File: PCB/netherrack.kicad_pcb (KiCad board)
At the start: 4 copper layers, 100 x 100 mm, 67 parts, among them J1 Conn_01x04, J11 USB_C_Receptacle_USB2.0, J12 USB3_A, J14 JST_SHBM04B-SRSS-TB, J2 Conn_02x07_Odd_Even, J22 690-019-298-412, J4 Bus_M.2_Socket_M, J6 THD-02-R, J7 Micro_SD_Card_Det, J9 THD-02-R, SW1 Right angle Tact button, U1 TPD4EUSB30, U12 RT9742SNGV, U18 RT9742GGJ5, U2 TPD4EUSB30, U3 MagJack-A70-112-331N126, U6 AP22653W6, U7 ASEK-32.768KHZ-L-R-T, U8 AP3441SHE-7B

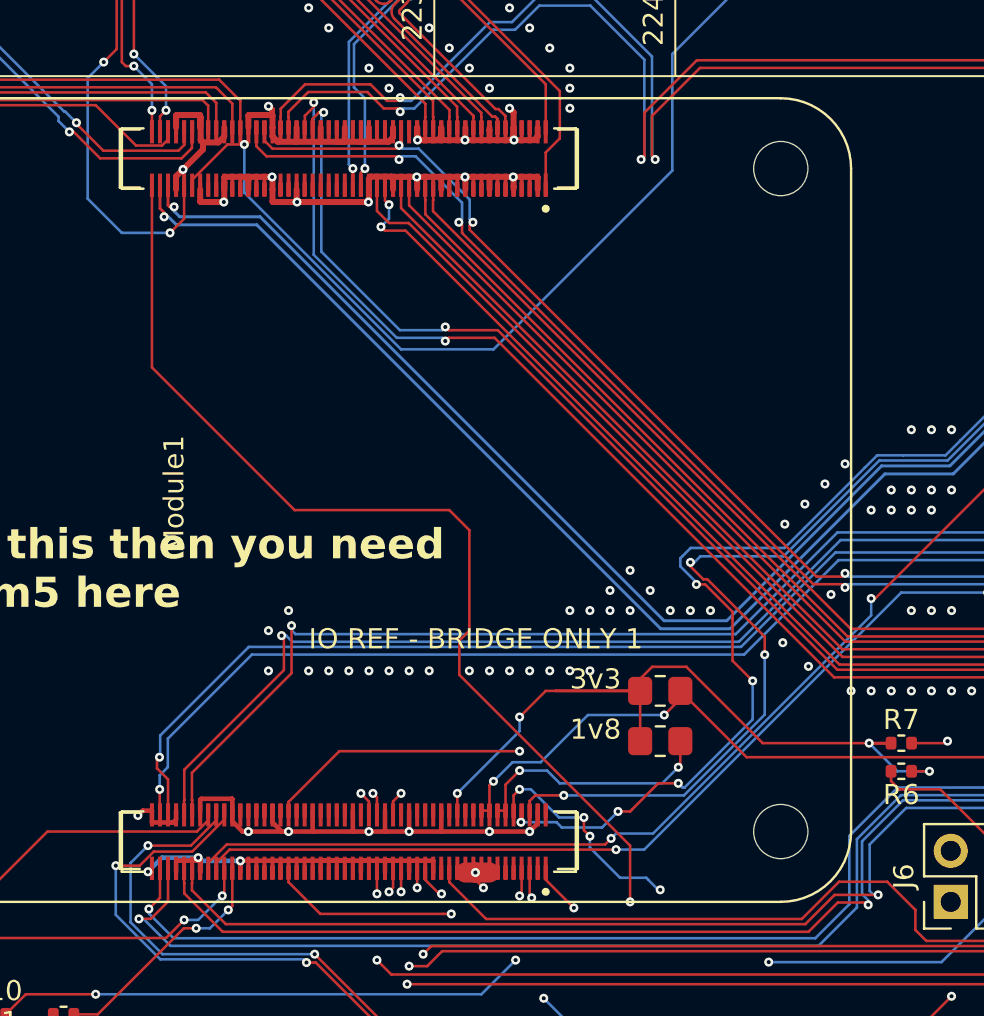
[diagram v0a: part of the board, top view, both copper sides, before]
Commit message: Update completed PCB
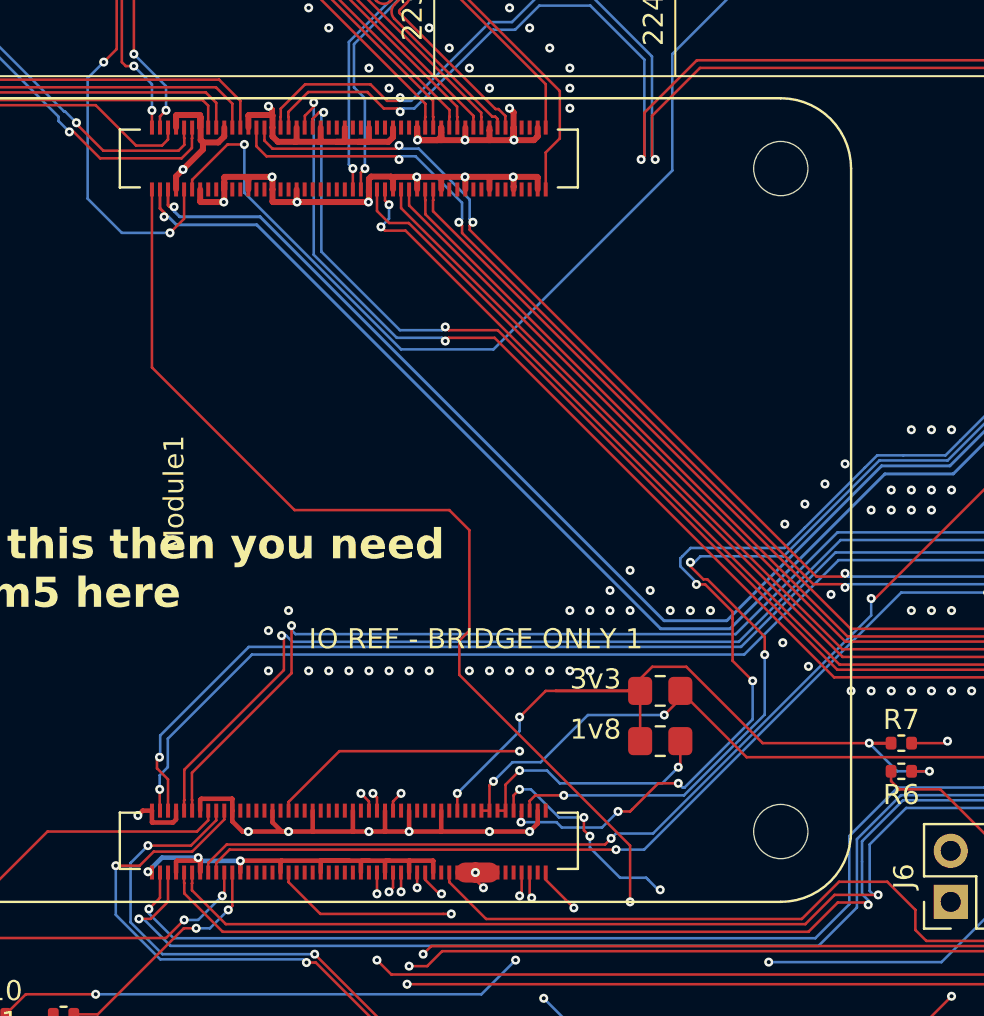
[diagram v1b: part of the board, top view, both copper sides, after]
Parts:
- removed REF** (x2): AMPHENOL_10164227-1001A1RLF, cm5conn:AMPHENOL_10164227-1001A1RLF

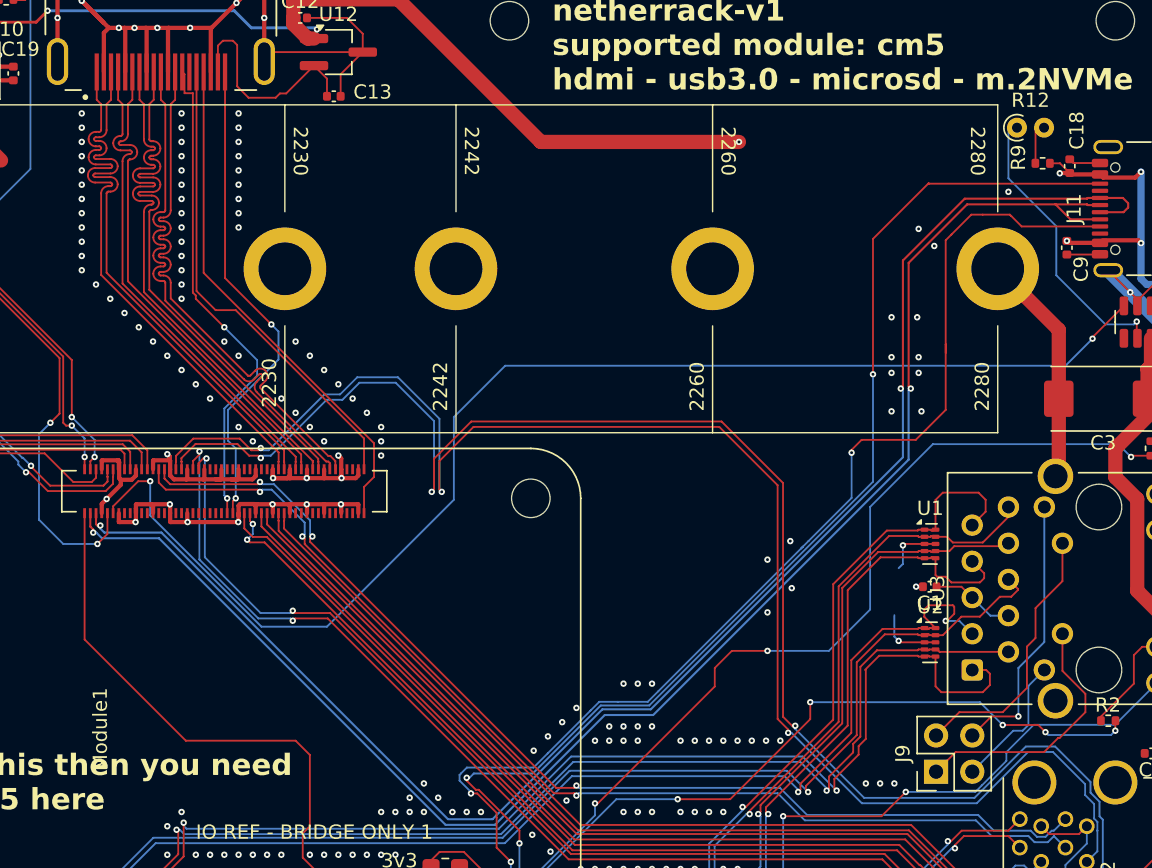
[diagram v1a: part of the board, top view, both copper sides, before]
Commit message: Submission commit
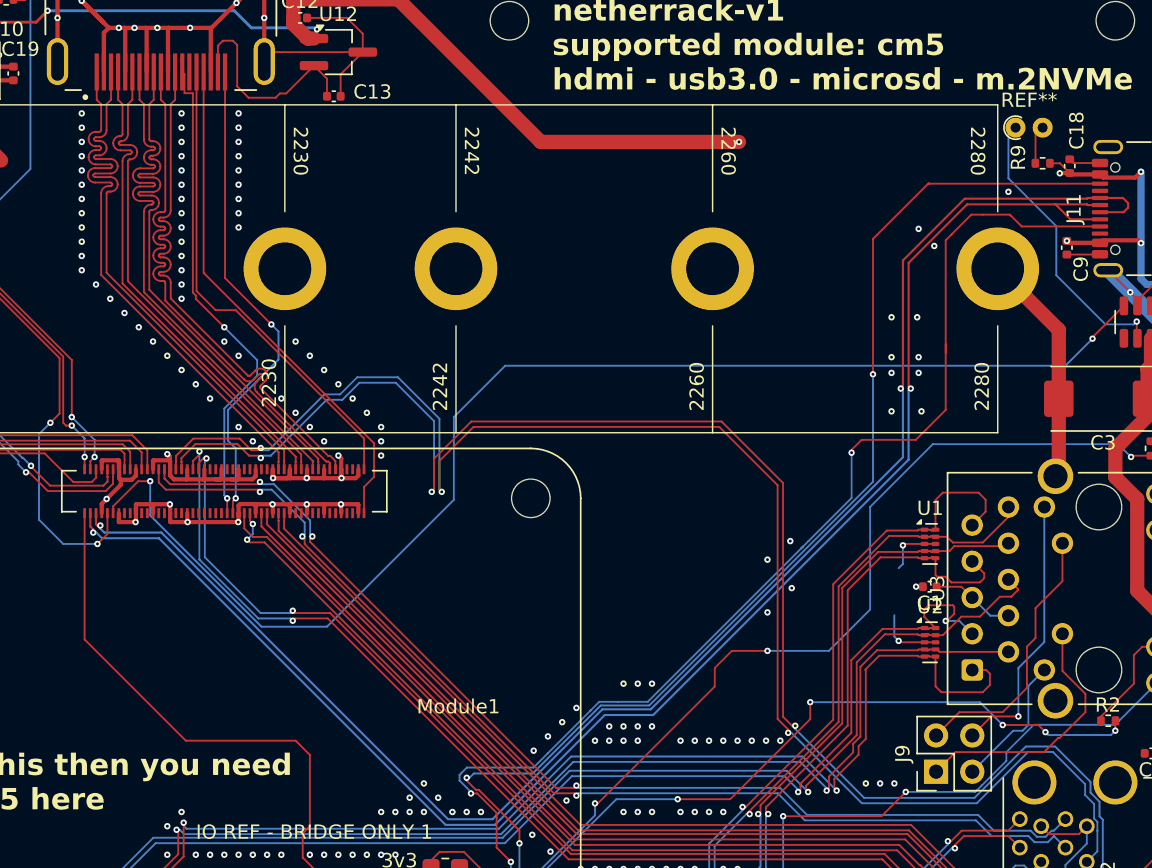
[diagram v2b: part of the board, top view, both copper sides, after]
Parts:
- removed R12: 15K 1%, Resistor_THT:R_Axial_DIN0204_L3.6mm_D1.6mm_P1.90mm_Vertical
- added REF**: R_Axial_DIN0204_L3.6mm_D1.6mm_P1.90mm_Vertical, Resistor_THT:R_Axial_DIN0204_L3.6mm_D1.6mm_P1.90mm_Vertical, F.Cu at (160.5, 60.0)
- D3: value LED Green -> LED
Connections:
- Module1 pad 1: (no net) -> GND
- Module1 pad 10: (no net) -> /GPIO (Ethernet, SD_CARD for CM5L)/TRD0_N
- Module1 pad 100: (no net) -> /GPIO (Ethernet, SD_CARD for CM5L)/CAM_GPIO1
- Module1 pad 101: (no net) -> /GPIO (Ethernet, SD_CARD for CM5L)/USBOTG
- Module1 pad 102: (no net) -> /Highspeed (USB, HDMI)/PCIE_nCLKREQ
- Module1 pad 103: (no net) -> /USB2_N
- Module1 pad 104: (no net) -> /Highspeed (USB, HDMI)/PCIE_nWAKE
- Module1 pad 105: (no net) -> /USB2_P
- Module1 pad 106: (no net) -> /Highspeed (USB, HDMI)/PCIE_PWR_EN
- Module1 pad 107: (no net) -> GND
- Module1 pad 108: (no net) -> GND
- Module1 pad 109: (no net) -> /Highspeed (USB, HDMI)/PCIE_nRST
- Module1 pad 11: (no net) -> /GPIO (Ethernet, SD_CARD for CM5L)/TRD2_P
- Module1 pad 110: (no net) -> /Highspeed (USB, HDMI)/PCIE_CLK_P
- Module1 pad 111: (no net) -> /Highspeed (USB, HDMI)/VBUS_EN
- Module1 pad 112: (no net) -> /Highspeed (USB, HDMI)/PCIE_CLK_N
- Module1 pad 113: (no net) -> GND
- Module1 pad 114: (no net) -> GND
- Module1 pad 115: (no net) -> /Highspeed (USB, HDMI)/DPHY0_D0_N
- Module1 pad 116: (no net) -> /Highspeed (USB, HDMI)/PCIE_RX_P
- Module1 pad 117: (no net) -> /Highspeed (USB, HDMI)/DPHY0_D0_P
- Module1 pad 118: (no net) -> /Highspeed (USB, HDMI)/PCIE_RX_N
- Module1 pad 119: (no net) -> GND
- Module1 pad 12: (no net) -> /GPIO (Ethernet, SD_CARD for CM5L)/TRD0_P
- Module1 pad 120: (no net) -> GND
- Module1 pad 121: (no net) -> /Highspeed (USB, HDMI)/DPHY0_D1_N
- Module1 pad 122: (no net) -> /Highspeed (USB, HDMI)/PCIE_TX_P
- Module1 pad 123: (no net) -> /Highspeed (USB, HDMI)/DPHY0_D1_P
- Module1 pad 124: (no net) -> /Highspeed (USB, HDMI)/PCIE_TX_N
- Module1 pad 125: (no net) -> GND
- Module1 pad 126: (no net) -> GND
- Module1 pad 127: (no net) -> /Highspeed (USB, HDMI)/DPHY0_C_N
- Module1 pad 128: (no net) -> /Highspeed (USB, HDMI)/USB3-0-RX_N
- Module1 pad 129: (no net) -> /Highspeed (USB, HDMI)/DPHY0_C_P
- Module1 pad 13: (no net) -> GND
- Module1 pad 130: (no net) -> /Highspeed (USB, HDMI)/USB3-0-RX_P
- Module1 pad 131: (no net) -> GND
- Module1 pad 132: (no net) -> GND
- Module1 pad 133: (no net) -> /Highspeed (USB, HDMI)/DPHY0_D2_N
- Module1 pad 134: (no net) -> /Highspeed (USB, HDMI)/USB3-0-D_P
- Module1 pad 135: (no net) -> /Highspeed (USB, HDMI)/DPHY0_D2_P
- Module1 pad 136: (no net) -> /Highspeed (USB, HDMI)/USB3-0-D_N
- Module1 pad 137: (no net) -> GND
- Module1 pad 138: (no net) -> GND
- Module1 pad 139: (no net) -> /Highspeed (USB, HDMI)/DPHY0_D3_N
- Module1 pad 14: (no net) -> GND
- Module1 pad 140: (no net) -> /Highspeed (USB, HDMI)/USB3-0-TX_N
- Module1 pad 141: (no net) -> /Highspeed (USB, HDMI)/DPHY0_D3_P
- Module1 pad 142: (no net) -> /Highspeed (USB, HDMI)/USB3-0-TX_P
- Module1 pad 143: (no net) -> /Highspeed (USB, HDMI)/HDMI1_HOTPLUG
- Module1 pad 144: (no net) -> GND
- Module1 pad 145: (no net) -> /Highspeed (USB, HDMI)/HDMI1_SDA
- Module1 pad 146: (no net) -> /Highspeed (USB, HDMI)/HDMI1_D2_P
- Module1 pad 147: (no net) -> /Highspeed (USB, HDMI)/HDMI1_SCL
- Module1 pad 148: (no net) -> /Highspeed (USB, HDMI)/HDMI1_D2_N
- Module1 pad 149: (no net) -> /Highspeed (USB, HDMI)/HDMI1_CEC
- Module1 pad 15: (no net) -> /GPIO (Ethernet, SD_CARD for CM5L)/ETH_LEDY
- Module1 pad 150: (no net) -> GND
- Module1 pad 151: (no net) -> /Highspeed (USB, HDMI)/HDMI0_CEC
- Module1 pad 152: (no net) -> /Highspeed (USB, HDMI)/HDMI1_D1_P
- Module1 pad 153: (no net) -> /Highspeed (USB, HDMI)/HDMI0_HOTPLUG
- Module1 pad 154: (no net) -> /Highspeed (USB, HDMI)/HDMI1_D1_N
- Module1 pad 155: (no net) -> GND
- Module1 pad 156: (no net) -> GND
- Module1 pad 157: (no net) -> /Highspeed (USB, HDMI)/USB3-1-RX_N
- Module1 pad 158: (no net) -> /Highspeed (USB, HDMI)/HDMI1_D0_P
- Module1 pad 159: (no net) -> /Highspeed (USB, HDMI)/USB3-1-RX_P
- Module1 pad 16: (no net) -> /GPIO (Ethernet, SD_CARD for CM5L)/TACHO
- Module1 pad 160: (no net) -> /Highspeed (USB, HDMI)/HDMI1_D0_N
- Module1 pad 161: (no net) -> GND
- Module1 pad 162: (no net) -> GND
- Module1 pad 163: (no net) -> /Highspeed (USB, HDMI)/USB3-1-D_P
- Module1 pad 164: (no net) -> /Highspeed (USB, HDMI)/HDMI1_CK_P
- Module1 pad 165: (no net) -> /Highspeed (USB, HDMI)/USB3-1-D_N
- Module1 pad 166: (no net) -> /Highspeed (USB, HDMI)/HDMI1_CK_N
- Module1 pad 167: (no net) -> GND
- Module1 pad 168: (no net) -> GND
- Module1 pad 169: (no net) -> /Highspeed (USB, HDMI)/USB3-1-TX_N
- Module1 pad 17: (no net) -> /GPIO (Ethernet, SD_CARD for CM5L)/ETH_LEDG
- Module1 pad 170: (no net) -> /Highspeed (USB, HDMI)/HDMI0_D2_P
- Module1 pad 171: (no net) -> /Highspeed (USB, HDMI)/USB3-1-TX_P
- Module1 pad 172: (no net) -> /Highspeed (USB, HDMI)/HDMI0_D2_N
- Module1 pad 173: (no net) -> GND
- Module1 pad 174: (no net) -> GND
- Module1 pad 175: (no net) -> /Highspeed (USB, HDMI)/DPHY1_D0_N
- Module1 pad 176: (no net) -> /Highspeed (USB, HDMI)/HDMI0_D1_P
- Module1 pad 177: (no net) -> /Highspeed (USB, HDMI)/DPHY1_D0_P
- Module1 pad 178: (no net) -> /Highspeed (USB, HDMI)/HDMI0_D1_N
- Module1 pad 179: (no net) -> GND
- Module1 pad 18: (no net) -> /GPIO (Ethernet, SD_CARD for CM5L)/SYNC_OUT
- Module1 pad 180: (no net) -> GND
- Module1 pad 181: (no net) -> /Highspeed (USB, HDMI)/DPHY1_D1_N
- Module1 pad 182: (no net) -> /Highspeed (USB, HDMI)/HDMI0_D0_P
- Module1 pad 183: (no net) -> /Highspeed (USB, HDMI)/DPHY1_D1_P
- Module1 pad 184: (no net) -> /Highspeed (USB, HDMI)/HDMI0_D0_N
- Module1 pad 185: (no net) -> GND
- Module1 pad 186: (no net) -> GND
- Module1 pad 187: (no net) -> /Highspeed (USB, HDMI)/DPHY1_C_N
- Module1 pad 188: (no net) -> /Highspeed (USB, HDMI)/HDMI0_CK_P
- Module1 pad 189: (no net) -> /Highspeed (USB, HDMI)/DPHY1_C_P
- Module1 pad 19: (no net) -> /GPIO (Ethernet, SD_CARD for CM5L)/PWM
- Module1 pad 190: (no net) -> /Highspeed (USB, HDMI)/HDMI0_CK_N
- Module1 pad 191: (no net) -> GND
- Module1 pad 192: (no net) -> GND
- Module1 pad 193: (no net) -> /Highspeed (USB, HDMI)/DPHY1_D2_N
- Module1 pad 194: (no net) -> /Highspeed (USB, HDMI)/DPHY1_D3_N
- Module1 pad 195: (no net) -> /Highspeed (USB, HDMI)/DPHY1_D2_P
- Module1 pad 196: (no net) -> /Highspeed (USB, HDMI)/DPHY1_D3_P
- Module1 pad 197: (no net) -> GND
- Module1 pad 198: (no net) -> GND
- Module1 pad 199: (no net) -> /Highspeed (USB, HDMI)/HDMI0_SDA
- Module1 pad 2: (no net) -> GND
- Module1 pad 20: (no net) -> /GPIO (Ethernet, SD_CARD for CM5L)/EEPROM_nWP
- Module1 pad 200: (no net) -> /Highspeed (USB, HDMI)/HDMI0_SCL
- Module1 pad 21: (no net) -> Net-(Module1A-LED_nACT)
- Module1 pad 22: (no net) -> GND
- Module1 pad 23: (no net) -> GND
- Module1 pad 24: (no net) -> /GPIO (Ethernet, SD_CARD for CM5L)/GPIO26
- Module1 pad 25: (no net) -> /GPIO (Ethernet, SD_CARD for CM5L)/GPIO21
- Module1 pad 26: (no net) -> /GPIO (Ethernet, SD_CARD for CM5L)/GPIO19
- Module1 pad 27: (no net) -> /GPIO (Ethernet, SD_CARD for CM5L)/GPIO20
- Module1 pad 28: (no net) -> /GPIO (Ethernet, SD_CARD for CM5L)/GPIO13
- Module1 pad 29: (no net) -> /GPIO (Ethernet, SD_CARD for CM5L)/GPIO16
- Module1 pad 3: (no net) -> /GPIO (Ethernet, SD_CARD for CM5L)/TRD3_P
- Module1 pad 30: (no net) -> /GPIO (Ethernet, SD_CARD for CM5L)/GPIO6
- Module1 pad 31: (no net) -> /GPIO (Ethernet, SD_CARD for CM5L)/GPIO12
- Module1 pad 32: (no net) -> GND
- Module1 pad 33: (no net) -> GND
- Module1 pad 34: (no net) -> /GPIO (Ethernet, SD_CARD for CM5L)/GPIO5
- Module1 pad 35: (no net) -> /GPIO (Ethernet, SD_CARD for CM5L)/ID_SC
- Module1 pad 36: (no net) -> /GPIO (Ethernet, SD_CARD for CM5L)/ID_SD
- Module1 pad 37: (no net) -> /GPIO (Ethernet, SD_CARD for CM5L)/GPIO7
- Module1 pad 38: (no net) -> /GPIO (Ethernet, SD_CARD for CM5L)/GPIO11
- Module1 pad 39: (no net) -> /GPIO (Ethernet, SD_CARD for CM5L)/GPIO8
- Module1 pad 4: (no net) -> /GPIO (Ethernet, SD_CARD for CM5L)/TRD1_P
- Module1 pad 40: (no net) -> /GPIO (Ethernet, SD_CARD for CM5L)/GPIO9
- Module1 pad 41: (no net) -> /GPIO (Ethernet, SD_CARD for CM5L)/GPIO25
- Module1 pad 42: (no net) -> GND
- Module1 pad 43: (no net) -> GND
- Module1 pad 44: (no net) -> /GPIO (Ethernet, SD_CARD for CM5L)/GPIO10
- Module1 pad 45: (no net) -> /GPIO (Ethernet, SD_CARD for CM5L)/GPIO24
- Module1 pad 46: (no net) -> /GPIO (Ethernet, SD_CARD for CM5L)/GPIO22
- Module1 pad 47: (no net) -> /GPIO (Ethernet, SD_CARD for CM5L)/GPIO23
- Module1 pad 48: (no net) -> /GPIO (Ethernet, SD_CARD for CM5L)/GPIO27
- Module1 pad 49: (no net) -> /GPIO (Ethernet, SD_CARD for CM5L)/GPIO18
- Module1 pad 5: (no net) -> /GPIO (Ethernet, SD_CARD for CM5L)/TRD3_N
- Module1 pad 50: (no net) -> /GPIO (Ethernet, SD_CARD for CM5L)/GPIO17
- Module1 pad 51: (no net) -> /GPIO (Ethernet, SD_CARD for CM5L)/GPIO15
- Module1 pad 52: (no net) -> GND
- Module1 pad 53: (no net) -> GND
- Module1 pad 54: (no net) -> /GPIO (Ethernet, SD_CARD for CM5L)/GPIO4
- Module1 pad 55: (no net) -> /GPIO (Ethernet, SD_CARD for CM5L)/GPIO14
- Module1 pad 56: (no net) -> /GPIO (Ethernet, SD_CARD for CM5L)/GPIO3
- Module1 pad 57: (no net) -> /GPIO (Ethernet, SD_CARD for CM5L)/SD_CLK
- Module1 pad 58: (no net) -> /GPIO (Ethernet, SD_CARD for CM5L)/GPIO2
- Module1 pad 59: (no net) -> GND
- Module1 pad 6: (no net) -> /GPIO (Ethernet, SD_CARD for CM5L)/TRD1_N
- Module1 pad 60: (no net) -> GND
- Module1 pad 61: (no net) -> /GPIO (Ethernet, SD_CARD for CM5L)/SD_DAT3
- Module1 pad 62: (no net) -> /GPIO (Ethernet, SD_CARD for CM5L)/SD_CMD
- Module1 pad 63: (no net) -> /GPIO (Ethernet, SD_CARD for CM5L)/SD_DAT0
- Module1 pad 64: (no net) -> unconnected-(Module1A-SD_DAT5-Pad64)
- Module1 pad 65: (no net) -> GND
- Module1 pad 66: (no net) -> GND
- Module1 pad 67: (no net) -> /GPIO (Ethernet, SD_CARD for CM5L)/SD_DAT1
- Module1 pad 68: (no net) -> unconnected-(Module1A-SD_DAT4-Pad68)
- Module1 pad 69: (no net) -> /GPIO (Ethernet, SD_CARD for CM5L)/SD_DAT2
- Module1 pad 7: (no net) -> GND
- Module1 pad 70: (no net) -> unconnected-(Module1A-SD_DAT7-Pad70)
- Module1 pad 71: (no net) -> GND
- Module1 pad 72: (no net) -> unconnected-(Module1A-SD_DAT6-Pad72)
- Module1 pad 73: (no net) -> unconnected-(Module1A-SD_VDD_Override-Pad73)
- Module1 pad 74: (no net) -> GND
- Module1 pad 75: (no net) -> /GPIO (Ethernet, SD_CARD for CM5L)/SD_PWR_ON
- Module1 pad 76: (no net) -> /GPIO (Ethernet, SD_CARD for CM5L)/VBAT
- Module1 pad 77: (no net) -> /+5v
- Module1 pad 78: (no net) -> /GPIO (Ethernet, SD_CARD for CM5L)/GPIO_VREF
- Module1 pad 79: (no net) -> /+5v
- Module1 pad 8: (no net) -> GND
- Module1 pad 80: (no net) -> /GPIO (Ethernet, SD_CARD for CM5L)/SCL0
- Module1 pad 81: (no net) -> /+5v
- Module1 pad 82: (no net) -> /GPIO (Ethernet, SD_CARD for CM5L)/SDA0
- Module1 pad 83: (no net) -> /+5v
- Module1 pad 84: (no net) -> /+3.3v
- Module1 pad 85: (no net) -> /+5v
- Module1 pad 86: (no net) -> /+3.3v
- Module1 pad 87: (no net) -> /+5v
- Module1 pad 88: (no net) -> /GPIO (Ethernet, SD_CARD for CM5L)/+1.8v
- Module1 pad 89: (no net) -> unconnected-(Module1A-WiFi_nDisable-Pad89)
- Module1 pad 9: (no net) -> /GPIO (Ethernet, SD_CARD for CM5L)/TRD2_N
- Module1 pad 90: (no net) -> /GPIO (Ethernet, SD_CARD for CM5L)/+1.8v
- Module1 pad 91: (no net) -> unconnected-(Module1A-BT_nDisable-Pad91)
- Module1 pad 92: (no net) -> /GPIO (Ethernet, SD_CARD for CM5L)/PWR_BUT
- Module1 pad 93: (no net) -> /GPIO (Ethernet, SD_CARD for CM5L)/nRPIBOOT
- Module1 pad 94: (no net) -> /CC1
- Module1 pad 95: (no net) -> /GPIO (Ethernet, SD_CARD for CM5L)/nPWR_LED
- Module1 pad 96: (no net) -> /CC2
- Module1 pad 97: (no net) -> /GPIO (Ethernet, SD_CARD for CM5L)/CAM_GPIO0
- Module1 pad 98: (no net) -> GND
- Module1 pad 99: (no net) -> /GPIO (Ethernet, SD_CARD for CM5L)/PMIC_ENABLE
